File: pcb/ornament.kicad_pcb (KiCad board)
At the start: 2 copper layers, 83.4 x 83.4 mm, 14 parts, among them J1 ICSP, U1 ATTINY2313-20MU

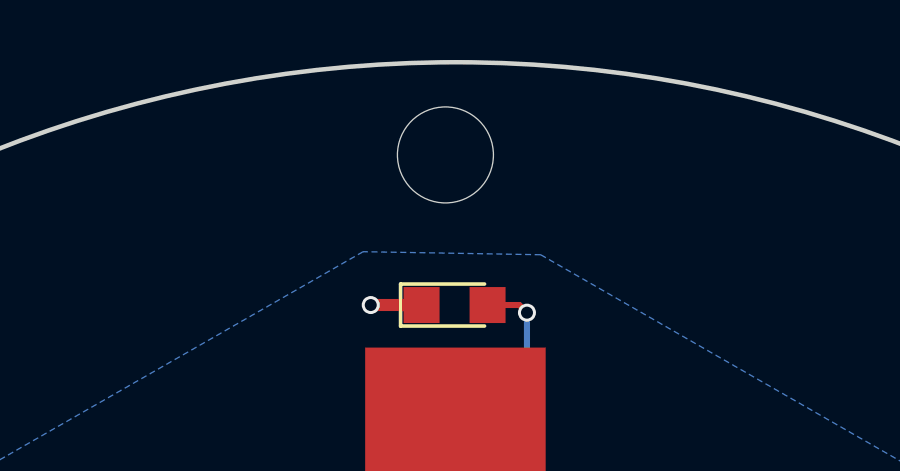
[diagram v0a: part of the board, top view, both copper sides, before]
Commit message: Add silkscreen.
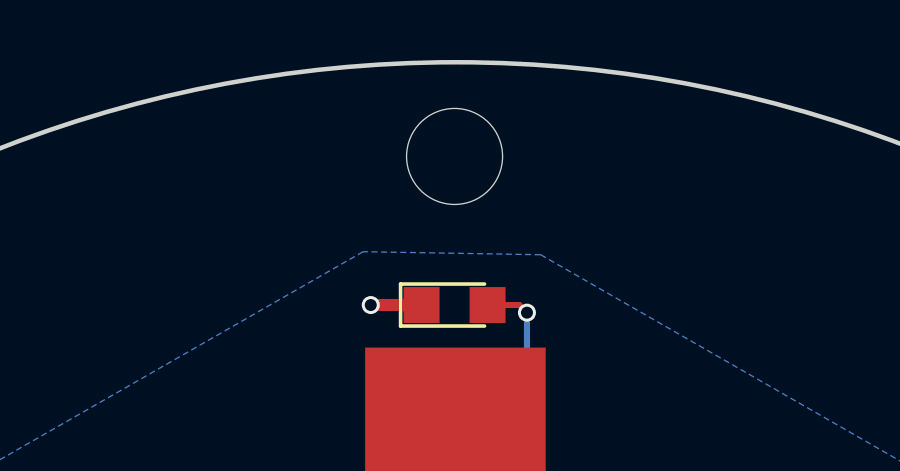
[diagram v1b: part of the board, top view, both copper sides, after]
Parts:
- moved REF** 0.31 mm to (69.8, 28.4)
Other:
- board text added: "2017"
- board text added: "David Tomaschik (@Matir)"
- board text added: "Merry Christmas"
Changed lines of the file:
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@@
     (links 35)
     (no_connects 0)
-    (area 28.103286 23.2222 131.665197 108.828114)
+    (area 28.103286 23.273 131.665197 108.828114)
     (thickness 1.6)
-    (drawings 2)
+    (drawings 5)
     (tracks 137)
     (zones 0)
@@
     (mod_text_size 1 1)
     (mod_text_width 0.15)
-    (pad_size 1.25 1.25)
+    (pad_size 17.780001 17.780001)
     (pad_drill 0)
     (pad_to_mask_clearance 0.2)
@@
     (visible_elements FFFFFF7F)
     (pcbplotparams
-      (layerselection 0x010d0_80000001)
+      (layerselection 0x010f0_80000001)
       (usegerberextensions true)
       (excludeedgelayer true)
@@
   )
   (module Mounting_Holes:MountingHole_3.2mm_M3 (layer F.Cu)
-    (at 69.5452 28.3972)
+    (at 69.85 28.448)
     (descr "Mounting Hole 3.2mm, no annular, M3")
     (tags "mounting hole 3.2mm no annular m3")
@@
   (module footprints:BAT_HLD (layer B.Cu)
     (at 69.977 63.5)
-    (fp_text reference BT1 (at 0 0) (layer B.SilkS)
-      (effects (font (size 1 1) (thickness 0.15)) (justify mirror))
-    )
-    (fp_text value Battery_Cell (at 0 0) (layer B.SilkS)
+    (fp_text reference BT1 (at 0 0) (layer B.SilkS) hide
+      (effects (font (size 1 1) (thickness 0.15)) (justify mirror))
+    )
+    (fp_text value Battery_Cell (at 0 0) (layer B.SilkS) hide
       (effects (font (size 1 1) (thickness 0.15)) (justify mirror))
     )
@@
       (net 1 VCC))
     (pad 2 smd circle (at 0 0) (size 17.780001 17.780001) (layers B.Cu B.Mask)
-      (net 2 GND))
+      (net 2 GND) (thermal_width 3) (thermal_gap 0.4))
+  )
+  (gr_text "David Tomaschik\n(@Matir)" (at 69.596 92.202) (layer B.SilkS)
+    (effects (font (size 2 2) (thickness 0.4)) (justify mirror))
+  )
+  (gr_text 2017 (at 70.104 46.355) (layer B.SilkS)
+    (effects (font (size 6 6) (thickness 1.2)) (justify mirror))
+  )
+  (gr_text "Merry Christmas" (at 69.596 38.735) (layer B.SilkS)
+    (effects (font (size 3 3) (thickness 0.6)) (justify mirror))
   )
   (dimension 83.312387 (width 0.3) (layer Dwgs.User)
